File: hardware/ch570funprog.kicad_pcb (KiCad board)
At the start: 2 copper layers, 34.3 x 10.9 mm, 25 parts, among them J1 USB_C_Receptacle_USB2.0, J2 PGM, Q1 PMOS-SI2301CDS-T1-GE3, U1 USBPROT, U2 AMS1117-3.3, U3 CH570Q, Y1 32M

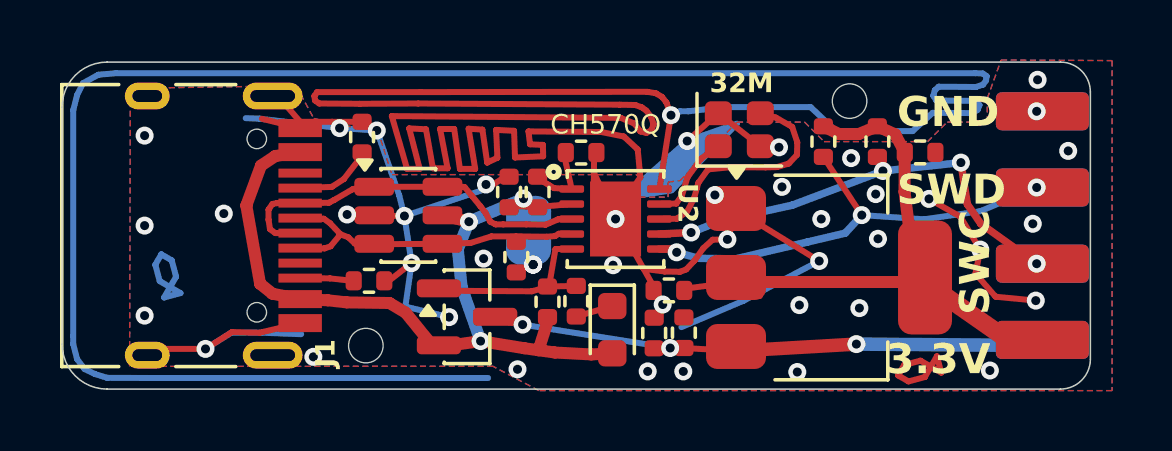
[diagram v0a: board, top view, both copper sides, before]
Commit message: Bump design
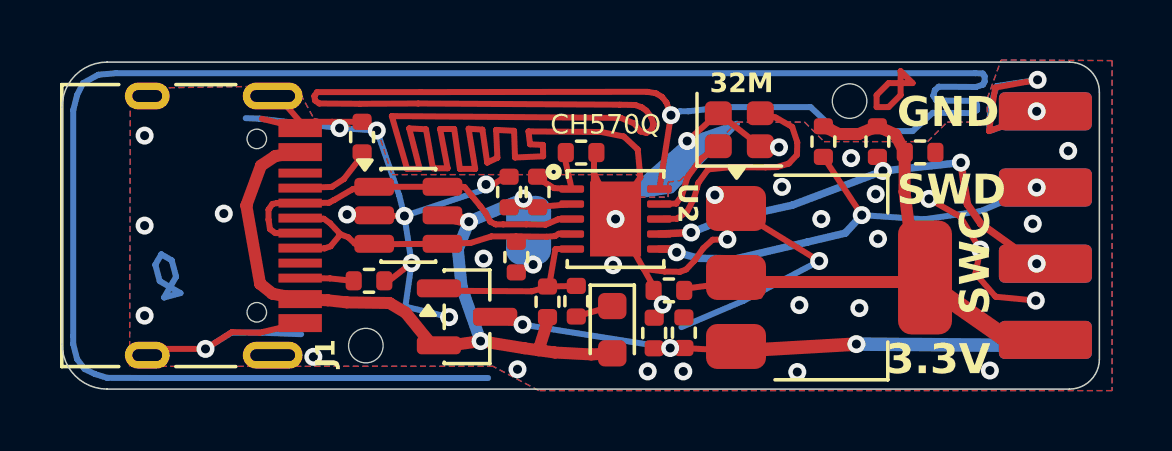
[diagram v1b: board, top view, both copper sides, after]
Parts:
- moved J2 0.10 mm to (151.3, 82.3)
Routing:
- net GND: track 192.9 -> 202.5 mm
- net Net-(JP1-A): vias 2 -> 1
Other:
- board size 34.3 x 10.9 mm -> 34.6 x 10.9 mm
